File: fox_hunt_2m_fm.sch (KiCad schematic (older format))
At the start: 19 parts, among them J1 I/O 1, J2 I/O 2, J3 BATT, J4 Ext Wire Ant, Q1 BSS138K, U1 MAX2606, U2 SMA3107

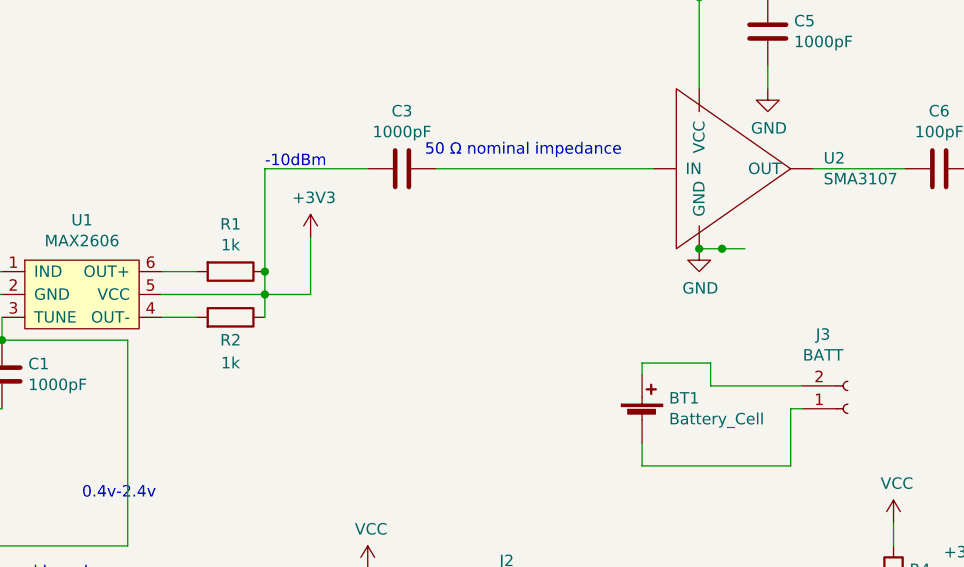
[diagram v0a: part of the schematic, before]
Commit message: Rev B
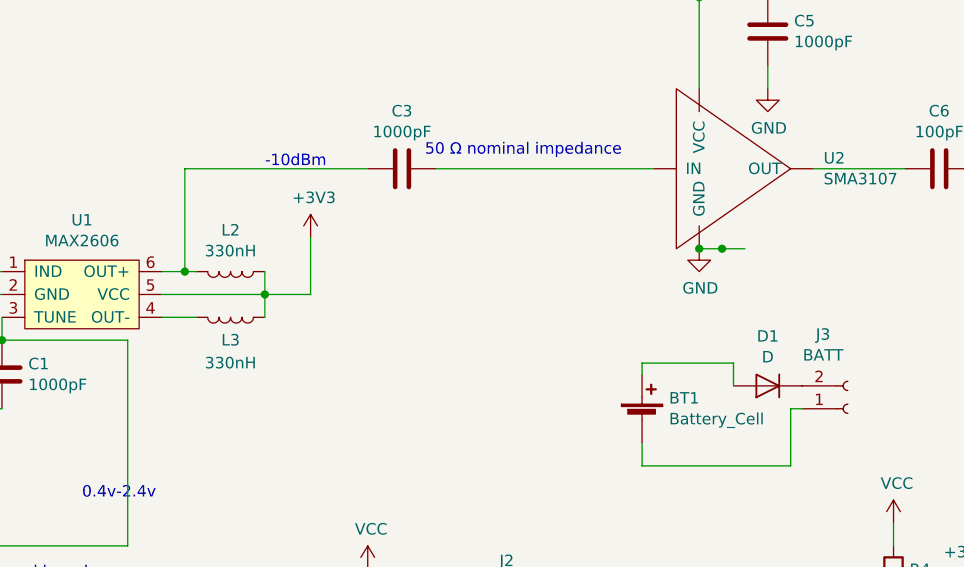
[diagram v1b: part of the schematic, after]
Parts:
- removed R1, R2: 1k, Resistor_SMD:R_1206_3216Metric_Pad1.30x1.75mm_HandSolder, symbol Device:R
- added D1: D, Diode_THT:D_DO-35_SOD27_P7.62mm_Horizontal, symbol Device:D
- added L2, L3: 330nH, Inductor_SMD:L_1008_2520Metric, symbol Device:L
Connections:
- net +3V3: now also L2.1, L3.1; no longer C3.2
- net at U1.4 (OUT-): now also L3.2
- net at U1.6 (OUT+): now also C3.2, L2.2
- net at J3.2 (Pin_2): now also D1.1 (K); no longer BT1.1 (+)
- new net: BT1.1 (+), D1.2 (A)
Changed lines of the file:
@@
 Wire Wire Line
 	4300 3300 4300 3700
-$Comp
-L Device:R R2
-U 1 1 607D1A99
-P 5450 3400
-F 0 "R2" V 5350 3400 50  0000 C CNN
-F 1 "1k" V 5250 3400 50  0000 C CNN
-F 2 "Resistor_SMD:R_1206_3216Metric_Pad1.30x1.75mm_HandSolder" V 5380 3400 50  0001 C CNN
-F 3 "~" H 5450 3400 50  0001 C CNN
-	1    5450 3400
-	0    1    -1   0
-$EndComp
-$Comp
-L Device:R R1
-U 1 1 607D264D
-P 5450 3200
-F 0 "R1" V 5243 3200 50  0000 C CNN
-F 1 "1k" V 5334 3200 50  0000 C CNN
-F 2 "Resistor_SMD:R_1206_3216Metric_Pad1.30x1.75mm_HandSolder" V 5380 3200 50  0001 C CNN
-F 3 "~" H 5450 3200 50  0001 C CNN
-	1    5450 3200
-	0    1    1    0
-$EndComp
-Wire Wire Line
-	5150 3200 5300 3200
+Wire Wire Line
+	5150 3200 5250 3200
 Wire Wire Line
 	5150 3400 5300 3400
 Wire Wire Line
-	5150 3300 5600 3300
-Wire Wire Line
-	5600 3300 5600 3200
-Wire Wire Line
-	5600 3300 5600 3400
-Connection ~ 5600 3300
-Wire Wire Line
 	5800 3050 5800 3300
-Wire Wire Line
-	5800 3300 5600 3300
 Wire Wire Line
 	4100 3700 4300 3700
@@
 	0    1    1    0
 $EndComp
-Wire Wire Line
-	5600 3200 5600 2750
-Wire Wire Line
-	5600 2750 6050 2750
-Connection ~ 5600 3200
 Text Notes 6300 2700 0    50   ~ 0
 50 Ω nominal impedance
@@
 	7250 3650 7250 3600
 Wire Wire Line
-	7250 3600 7550 3600
-Wire Wire Line
-	7550 3600 7550 3700
-Wire Wire Line
-	7550 3700 7950 3700
+	7250 3600 7650 3600
 Wire Wire Line
 	7950 3800 7900 3800
@@
 Wire Wire Line
 	7650 4950 8050 4950
+Wire Wire Line
+	5150 3300 5600 3300
+$Comp
+L Device:L L2
+U 1 1 60B15913
+P 5450 3200
+F 0 "L2" V 5269 3200 50  0000 C CNN
+F 1 "330nH" V 5360 3200 50  0000 C CNN
+F 2 "Inductor_SMD:L_1008_2520Metric" H 5450 3200 50  0001 C CNN
+F 3 "~" H 5450 3200 50  0001 C CNN
+	1    5450 3200
+	0    1    1    0
+$EndComp
+$Comp
+L Device:L L3
+U 1 1 60B161F4
+P 5450 3400
+F 0 "L3" V 5550 3400 50  0000 C CNN
+F 1 "330nH" V 5650 3400 50  0000 C CNN
+F 2 "Inductor_SMD:L_1008_2520Metric" H 5450 3400 50  0001 C CNN
+F 3 "~" H 5450 3400 50  0001 C CNN
+	1    5450 3400
+	0    1    1    0
+$EndComp
+Wire Wire Line
+	5600 3200 5600 3300
+Connection ~ 5600 3300
+Wire Wire Line
+	5600 3300 5800 3300
+Wire Wire Line
+	5600 3400 5600 3300
+Wire Wire Line
+	5250 2750 5250 3200
+Wire Wire Line
+	5250 2750 6050 2750
+Connection ~ 5250 3200
+Wire Wire Line
+	5250 3200 5300 3200
+$Comp
+L Device:D D1
+U 1 1 60B2CDBE
+P 7800 3700
+F 0 "D1" H 7800 3483 50  0000 C CNN
+F 1 "D" H 7800 3574 50  0000 C CNN
+F 2 "Diode_THT:D_DO-35_SOD27_P7.62mm_Horizontal" H 7800 3700 50  0001 C CNN
+F 3 "~" H 7800 3700 50  0001 C CNN
+	1    7800 3700
+	-1   0    0    1
+$EndComp
+Wire Wire Line
+	7650 3600 7650 3700
 $EndSCHEMATC

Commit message: Board and schematic Rev. C
Use IO line to directly power analog section.
Remove power MOSFET as it's not needed.
Add additional filter cap.
Rearrange PCB to account for above.
Add antenna length to silkscreen.
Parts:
- removed Q1: BSS138K, Package_TO_SOT_SMD:SOT-23, symbol Transistor_FET:BSS138
- removed R4: 15, Resistor_SMD:R_1206_3216Metric_Pad1.30x1.75mm_HandSolder, symbol Device:R
- added C7: 470pF, Capacitor_SMD:C_1206_3216Metric_Pad1.42x1.75mm_HandSolder, symbol Device:C
- U1: symbol vw:MAX260x -> fox_hunt_2m_fm-rescue:MAX260x-vw
- U2: symbol vw:SMA3107 -> fox_hunt_2m_fm-rescue:SMA3107-vw
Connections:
- net +3V3: now also C2.1, C4.1, R3.1, C7.1
- net GND: now also C7.2
- removed net VCC: C2.1, C4.1, J1.4 (Pin_4), J1.5 (Pin_5), J1.6 (Pin_6)
- no-connect marks 4 -> 8
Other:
- note added: "Decoupling and\nregulation is on\nthe digital board"
- note added: "Each leg approx\n20.5 inches"
- moved on the sheet: C2, C4
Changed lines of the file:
@@
 $EndDescr
 $Comp
-L vw:MAX260x U1
+L fox_hunt_2m_fm-rescue:MAX260x-vw U1
 U 1 1 607CF170
 P 4800 3300
@@
 L Device:C C2
 U 1 1 607D4142
-P 5300 4750
-F 0 "C2" H 5415 4796 50  0000 L CNN
-F 1 "0.1uF" H 5350 4700 50  0000 L CNN
-F 2 "Capacitor_SMD:C_1206_3216Metric_Pad1.33x1.80mm_HandSolder" H 5338 4600 50  0001 C CNN
-F 3 "~" H 5300 4750 50  0001 C CNN
-	1    5300 4750
-	1    0    0    -1
-$EndComp
-Wire Wire Line
-	5650 4550 5650 4600
-Wire Wire Line
-	5300 4600 5300 4550
-Wire Wire Line
-	5300 4550 5650 4550
+P 7650 5150
+F 0 "C2" H 7765 5196 50  0000 L CNN
+F 1 "0.1uF" H 7700 5100 50  0000 L CNN
+F 2 "Capacitor_SMD:C_1206_3216Metric_Pad1.33x1.80mm_HandSolder" H 7688 5000 50  0001 C CNN
+F 3 "~" H 7650 5150 50  0001 C CNN
+	1    7650 5150
+	1    0    0    -1
+$EndComp
+Wire Wire Line
+	8000 4950 8000 5000
+Wire Wire Line
+	7650 5000 7650 4950
+Wire Wire Line
+	7650 4950 8000 4950
 $Comp
 L power:GND #PWR0103
 U 1 1 607D4C59
-P 5500 5050
-F 0 "#PWR0103" H 5500 4800 50  0001 C CNN
-F 1 "GND" H 5505 4877 50  0000 C CNN
-F 2 "" H 5500 5050 50  0001 C CNN
-F 3 "" H 5500 5050 50  0001 C CNN
-	1    5500 5050
-	1    0    0    -1
-$EndComp
-Wire Wire Line
-	5300 4900 5500 4900
-Wire Wire Line
-	5500 5050 5500 4900
-Connection ~ 5500 4900
-Wire Wire Line
-	5500 4900 5650 4900
+P 7850 5450
+F 0 "#PWR0103" H 7850 5200 50  0001 C CNN
+F 1 "GND" H 7855 5277 50  0000 C CNN
+F 2 "" H 7850 5450 50  0001 C CNN
+F 3 "" H 7850 5450 50  0001 C CNN
+	1    7850 5450
+	1    0    0    -1
+$EndComp
+Wire Wire Line
+	7650 5300 7850 5300
+Wire Wire Line
+	7850 5450 7850 5300
+Connection ~ 7850 5300
+Wire Wire Line
+	7850 5300 8000 5300
 $Comp
 L Device:C C3
@@
 -10dBm
 $Comp
-L vw:SMA3107 U2
+L fox_hunt_2m_fm-rescue:SMA3107-vw U2
 U 1 1 607D77B1
 P 7600 2750
@@
 Text GLabel 4250 4400 0    50   Input ~ 0
 TUNE
-Text Notes 3950 4550 0    50   ~ 0
+Text Notes 5950 5250 0    50   ~ 0
 ATtiny212 external board
 Text Notes 8750 2650 0    50   ~ 0
@@
 $EndComp
 $Comp
-L power:VCC #PWR01
-U 1 1 607F8484
-P 6050 4500
-F 0 "#PWR01" H 6050 4350 50  0001 C CNN
-F 1 "VCC" H 6065 4673 50  0000 C CNN
-F 2 "" H 6050 4500 50  0001 C CNN
-F 3 "" H 6050 4500 50  0001 C CNN
-	1    6050 4500
-	1    0    0    -1
-$EndComp
-Wire Wire Line
-	6050 4500 6050 4550
-Wire Wire Line
-	6050 4850 6200 4850
-Wire Wire Line
-	6200 4750 6050 4750
-Connection ~ 6050 4750
-Wire Wire Line
-	6050 4750 6050 4850
-Wire Wire Line
-	6200 4650 6050 4650
-Connection ~ 6050 4650
-Wire Wire Line
-	6050 4650 6050 4750
-$Comp
 L power:GND #PWR02
 U 1 1 607FA951
@@
 NoConn ~ 6750 5150
 $Comp
-L Transistor_FET:BSS138 Q1
-U 1 1 608046BE
-P 8250 4950
-F 0 "Q1" H 8454 4996 50  0000 L CNN
-F 1 "BSS138K" H 8454 4905 50  0000 L CNN
-F 2 "Package_TO_SOT_SMD:SOT-23" H 8450 4875 50  0001 L CIN
-F 3 "https://www.onsemi.com/pub/Collateral/BSS138-D.PDF" H 8250 4950 50  0001 L CNN
-	1    8250 4950
-	1    0    0    -1
-$EndComp
-$Comp
 L power:+3V3 #PWR05
 U 1 1 6080B91D
-P 8650 4600
-F 0 "#PWR05" H 8650 4450 50  0001 C CNN
-F 1 "+3V3" H 8665 4773 50  0000 C CNN
-F 2 "" H 8650 4600 50  0001 C CNN
-F 3 "" H 8650 4600 50  0001 C CNN
-	1    8650 4600
-	1    0    0    -1
-$EndComp
-$Comp
-L Device:R R4
-U 1 1 6080D77A
-P 8350 4550
-F 0 "R4" H 8420 4596 50  0000 L CNN
-F 1 "15" H 8420 4505 50  0000 L CNN
-F 2 "Resistor_SMD:R_1206_3216Metric_Pad1.30x1.75mm_HandSolder" V 8280 4550 50  0001 C CNN
-F 3 "~" H 8350 4550 50  0001 C CNN
-	1    8350 4550
-	1    0    0    -1
-$EndComp
-Wire Wire Line
-	8350 4700 8650 4700
-Wire Wire Line
-	8650 4700 8650 4600
-$Comp
-L power:VCC #PWR03
-U 1 1 608129D5
-P 8350 4300
-F 0 "#PWR03" H 8350 4150 50  0001 C CNN
-F 1 "VCC" H 8365 4473 50  0000 C CNN
-F 2 "" H 8350 4300 50  0001 C CNN
-F 3 "" H 8350 4300 50  0001 C CNN
-	1    8350 4300
-	1    0    0    -1
-$EndComp
-Wire Wire Line
-	8350 4300 8350 4400
+P 7650 4850
+F 0 "#PWR05" H 7650 4700 50  0001 C CNN
+F 1 "+3V3" H 7665 5023 50  0000 C CNN
+F 2 "" H 7650 4850 50  0001 C CNN
+F 3 "" H 7650 4850 50  0001 C CNN
+	1    7650 4850
+	1    0    0    -1
+$EndComp
+Wire Wire Line
+	7650 4950 7650 4850
 $Comp
 L Device:R R3
@@
 Wire Wire Line
 	6750 4950 7350 4950
-Wire Wire Line
-	8350 4750 8350 4700
-Connection ~ 8350 4700
-$Comp
-L power:GND #PWR04
-U 1 1 6081A9EA
-P 8350 5350
-F 0 "#PWR04" H 8350 5100 50  0001 C CNN
-F 1 "GND" H 8355 5177 50  0000 C CNN
-F 2 "" H 8350 5350 50  0001 C CNN
-F 3 "" H 8350 5350 50  0001 C CNN
-	1    8350 5350
-	1    0    0    -1
-$EndComp
-Wire Wire Line
-	8350 5150 8350 5350
 $Comp
 L power:+3V3 #PWR0102
@@
 $EndComp
 Connection ~ 7500 2000
-Wire Wire Line
-	6050 4550 5650 4550
-Connection ~ 6050 4550
-Wire Wire Line
-	6050 4550 6050 4650
-Connection ~ 5650 4550
 $Comp
 L Connector_Generic:Conn_01x02 J4
@@
 Wire Wire Line
 	8900 2850 8950 2850
-$Comp
-L Device:C C4
-U 1 1 6082A2D3
-P 5650 4750
-F 0 "C4" H 5765 4796 50  0000 L CNN
-F 1 "1uF" H 5700 4700 50  0000 L CNN
-F 2 "Capacitor_SMD:C_1206_3216Metric_Pad1.33x1.80mm_HandSolder" H 5688 4600 50  0001 C CNN
-F 3 "~" H 5650 4750 50  0001 C CNN
-	1    5650 4750
-	1    0    0    -1
-$EndComp
-Wire Wire Line
-	7650 4950 8050 4950
 Wire Wire Line
 	5150 3300 5600 3300
@@
 Wire Wire Line
 	7650 3600 7650 3700
+Connection ~ 7650 4950
+$Comp
+L Device:C C4
+U 1 1 6082A2D3
+P 8000 5150
+F 0 "C4" H 8115 5196 50  0000 L CNN
+F 1 "1uF" H 8050 5100 50  0000 L CNN
+F 2 "Capacitor_SMD:C_1206_3216Metric_Pad1.33x1.80mm_HandSolder" H 8038 5000 50  0001 C CNN
+F 3 "~" H 8000 5150 50  0001 C CNN
+	1    8000 5150
+	1    0    0    -1
+$EndComp
+$Comp
+L Device:C C7
+U 1 1 60DDFC83
+P 8350 5150
+F 0 "C7" H 8465 5196 50  0000 L CNN
+F 1 "470pF" H 8400 5100 50  0000 L CNN
+F 2 "Capacitor_SMD:C_1206_3216Metric_Pad1.42x1.75mm_HandSolder" H 8388 5000 50  0001 C CNN
+F 3 "~" H 8350 5150 50  0001 C CNN
+	1    8350 5150
+	1    0    0    -1
+$EndComp
+Wire Wire Line
+	8000 5300 8350 5300
+Connection ~ 8000 5300
+Wire Wire Line
+	8000 4950 8350 4950
+Wire Wire Line
+	8350 4950 8350 5000
+Connection ~ 8000 4950
+Text Notes 7300 4200 0    50   ~ 0
+Decoupling and\nregulation is on\nthe digital board
+NoConn ~ 6200 4850
+NoConn ~ 6200 4750
+NoConn ~ 6200 4650
+NoConn ~ 3700 5350
+Text Notes 9100 3100 0    50   ~ 0
+Each leg approx\n20.5 inches
 $EndSCHEMATC
